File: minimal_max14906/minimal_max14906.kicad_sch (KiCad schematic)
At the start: 114 parts, among them J10 TBP02R2-381-02BE, J11 TBP02R2-381-02BE, J12 CLP-102-02-G-D-BE, J13 CLP-108-02-G-D-BE, J14 CLP-108-02-G-D-BE, J15 CLP-102-02-G-D-BE, J2 TBP02R2-381-02BE, J3 TBP02R2-381-02BE, J4 CLP-102-02-G-D-BE, J5 CLP-102-02-G-D-BE, J6 CLP-102-02-G-D-BE, J7 CLP-102-02-G-D-BE, J8 CLP-102-02-G-D-BE, Q1 -60.0 V, Q2 -60.0 V, Q3 -60.0 V, Q4 -60.0 V, Q5 100 V, Q6 100 V, U1 ADUM1252AUA+, U2 MAX22441CAEE+, U3 MAX22442CAEE+, U4 ADUM1252AUA+, U5 MAX14906ATM+, U6 ADUM1252AUA+

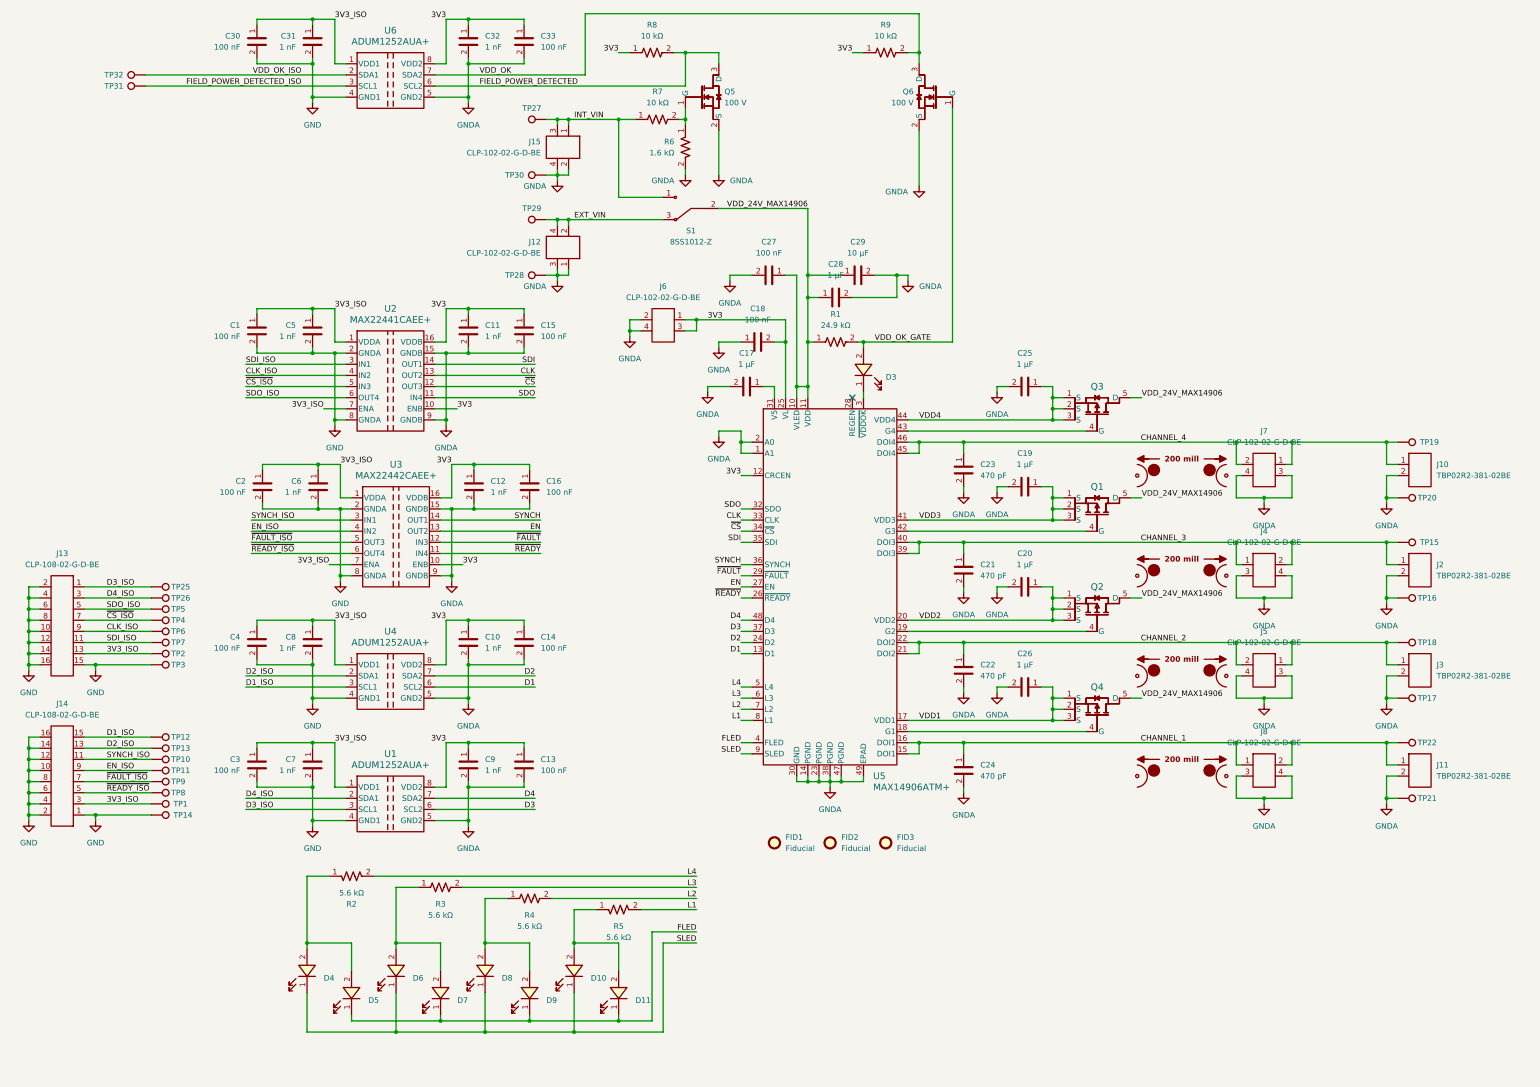
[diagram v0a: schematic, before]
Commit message: development backup
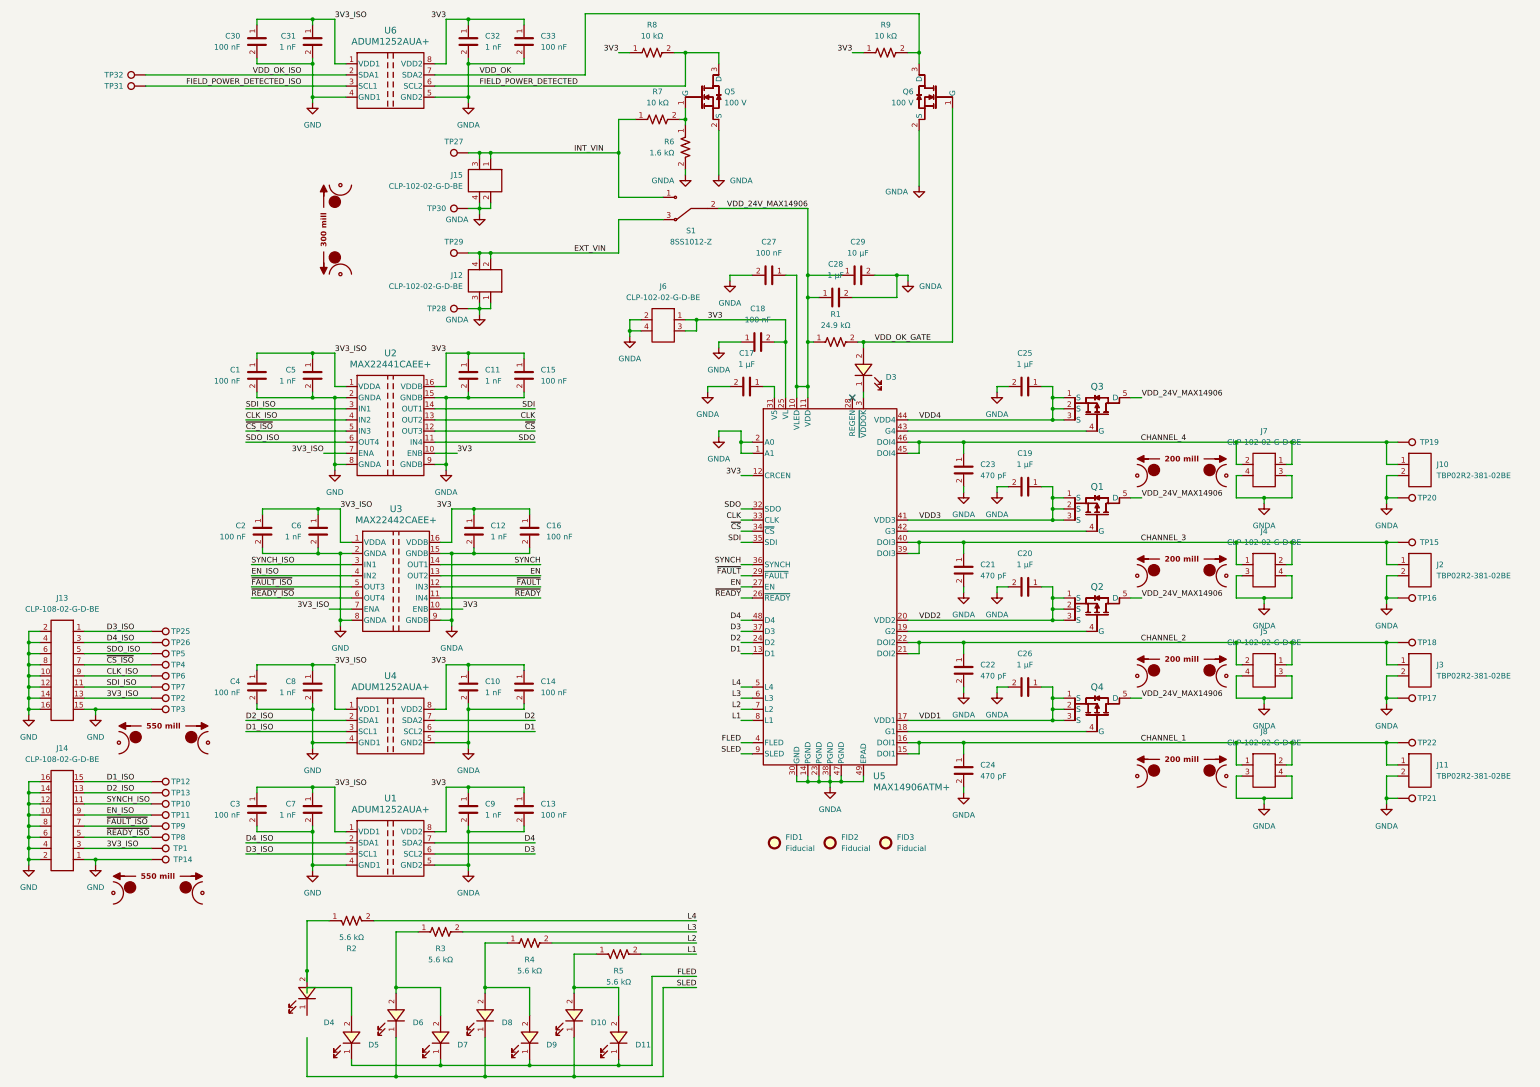
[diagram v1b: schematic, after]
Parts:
- added MB1, MB6: mouse-bite-50mil-550mil, mouse_bite_footprints:mouse-bite-50mil-550mil, symbol UNITED_MOUSE_BITES_DATA_BASE:mouse-bite-50mil-550mil
- added MB8: mouse-bite-50mil-300mil, mouse_bite_footprints:mouse-bite-50mil-300mil, symbol UNITED_MOUSE_BITES_DATA_BASE:mouse-bite-50mil-300mil
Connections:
- net SLED: no longer D4.1
- net at D4.2, R2.1: no longer D5.2
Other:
- moved on the sheet: C1, C10, C11, C12, C13, C14, C15, C16, C2, C3, C4, C5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
